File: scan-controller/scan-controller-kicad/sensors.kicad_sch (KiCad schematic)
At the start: 28 parts, among them CN5 Film End Eye, CN6 Shaft Eye, J2 Shaft Eye, J3 Film End Eye, Q5 SS8050, Q6 SS8050, U1 QRE1113, U2 QRE1113, U9 74LVC14

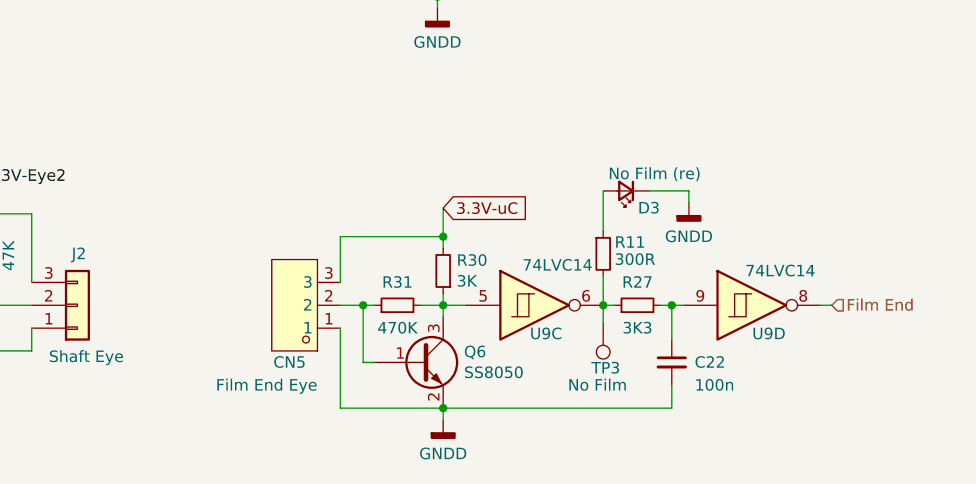
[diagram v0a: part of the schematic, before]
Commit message: Add C31 to U9 to form another low pass
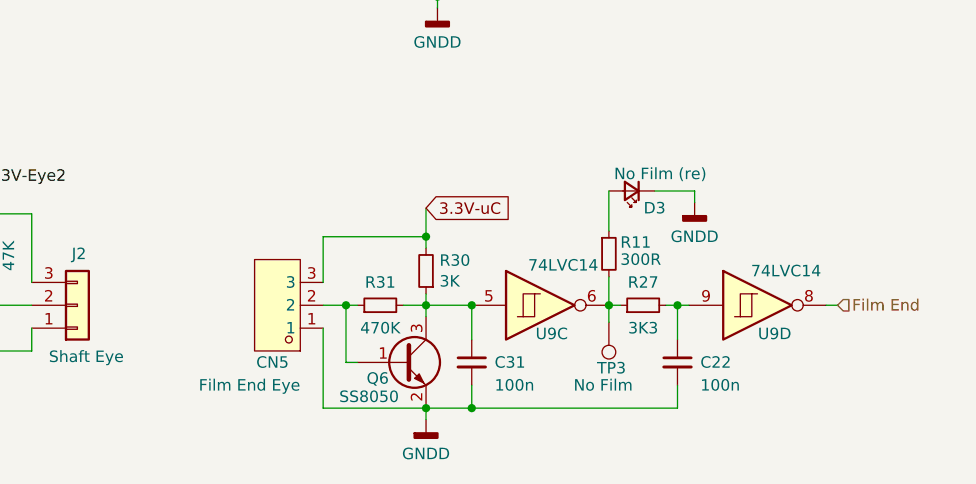
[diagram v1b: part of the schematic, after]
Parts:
- added C31: 100n, Capacitor_SMD:C_0805_2012Metric, symbol Device:C_Small
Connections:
- net GNDD: now also C31.2
- net at Q6.3 (C), R30.1, R31.2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: now also C31.1
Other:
- moved on the sheet: C22, CN5, D3, Q6, R11, R27, R30, R31, TP3, U9C, U9D

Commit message: reassigned customfootprints to now gobal library
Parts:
- R1, R3, R5, R6: footprint Peacemans_Footprints:R_0402_1005Metric-noref -> Peacemans_Teile:R_0402_1005Metric-noref
- TP10, TP3: footprint Peacemans_Footprints:TestPoint_THTPad_1.5x1.5mm_Drill0.7mm_named -> Peacemans_Teile:TestPoint_THTPad_1.5x1.5mm_Drill0.7mm_named
- U1, U2: footprint Peacemans_Footprints:QRE1113GR-slim -> Peacemans_Teile:QRE1113GR-slim
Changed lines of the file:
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@@
 			)
 		)
-		(property "Footprint" "Peacemans_Footprints:R_0402_1005Metric-noref"
+		(property "Footprint" "Peacemans_Teile:R_0402_1005Metric-noref"
 			(at 107.315 114.3 0)
 			(effects
@@
 			)
 		)
-		(property "Footprint" "Peacemans_Footprints:QRE1113GR-slim"
+		(property "Footprint" "Peacemans_Teile:QRE1113GR-slim"
 			(at 98.425 81.28 0)
 			(effects
@@
 			)
 		)
-		(property "Footprint" "Peacemans_Footprints:TestPoint_THTPad_1.5x1.5mm_Drill0.7mm_named"
+		(property "Footprint" "Peacemans_Teile:TestPoint_THTPad_1.5x1.5mm_Drill0.7mm_named"
 			(at 171.45 121.285 0)
 			(effects
@@
 			)
 		)
-		(property "Footprint" "Peacemans_Footprints:QRE1113GR-slim"
+		(property "Footprint" "Peacemans_Teile:QRE1113GR-slim"
 			(at 99.695 127 0)
 			(effects
@@
 			)
 		)
-		(property "Footprint" "Peacemans_Footprints:R_0402_1005Metric-noref"
+		(property "Footprint" "Peacemans_Teile:R_0402_1005Metric-noref"
 			(at 90.805 68.58 0)
 			(effects
@@
 			)
 		)
-		(property "Footprint" "Peacemans_Footprints:R_0402_1005Metric-noref"
+		(property "Footprint" "Peacemans_Teile:R_0402_1005Metric-noref"
 			(at 106.045 68.58 0)
 			(effects
@@
 			)
 		)
-		(property "Footprint" "Peacemans_Footprints:R_0402_1005Metric-noref"
+		(property "Footprint" "Peacemans_Teile:R_0402_1005Metric-noref"
 			(at 92.075 114.3 0)
 			(effects
@@
 			)
 		)
-		(property "Footprint" "Peacemans_Footprints:TestPoint_THTPad_1.5x1.5mm_Drill0.7mm_named"
+		(property "Footprint" "Peacemans_Teile:TestPoint_THTPad_1.5x1.5mm_Drill0.7mm_named"
 			(at 170.18 75.565 0)
 			(effects
